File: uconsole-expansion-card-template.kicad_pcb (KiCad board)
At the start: 2 copper layers, 35.8 x 77 mm, 21 parts, among them U1 UC EXPANSION, U2 Speaker, U3 Speaker

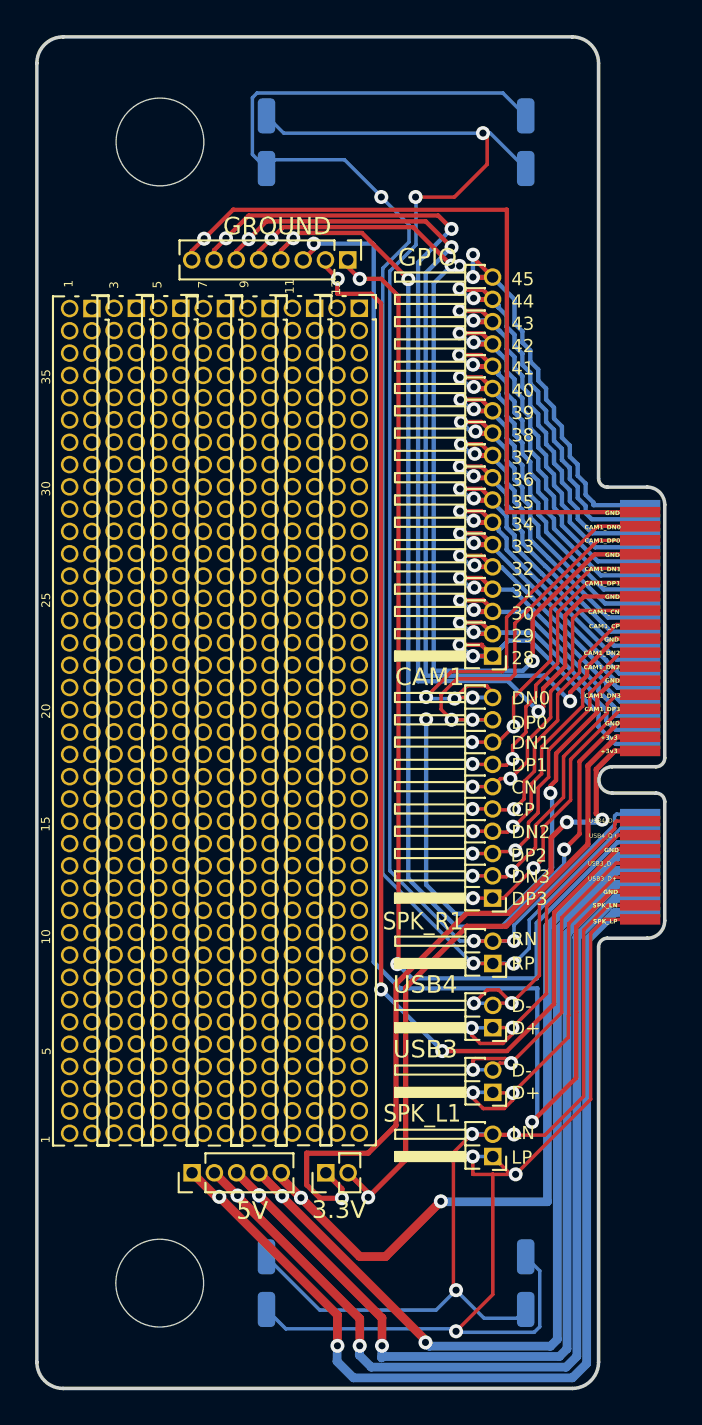
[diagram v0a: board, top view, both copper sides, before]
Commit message: Board 1.27mm passes to production!
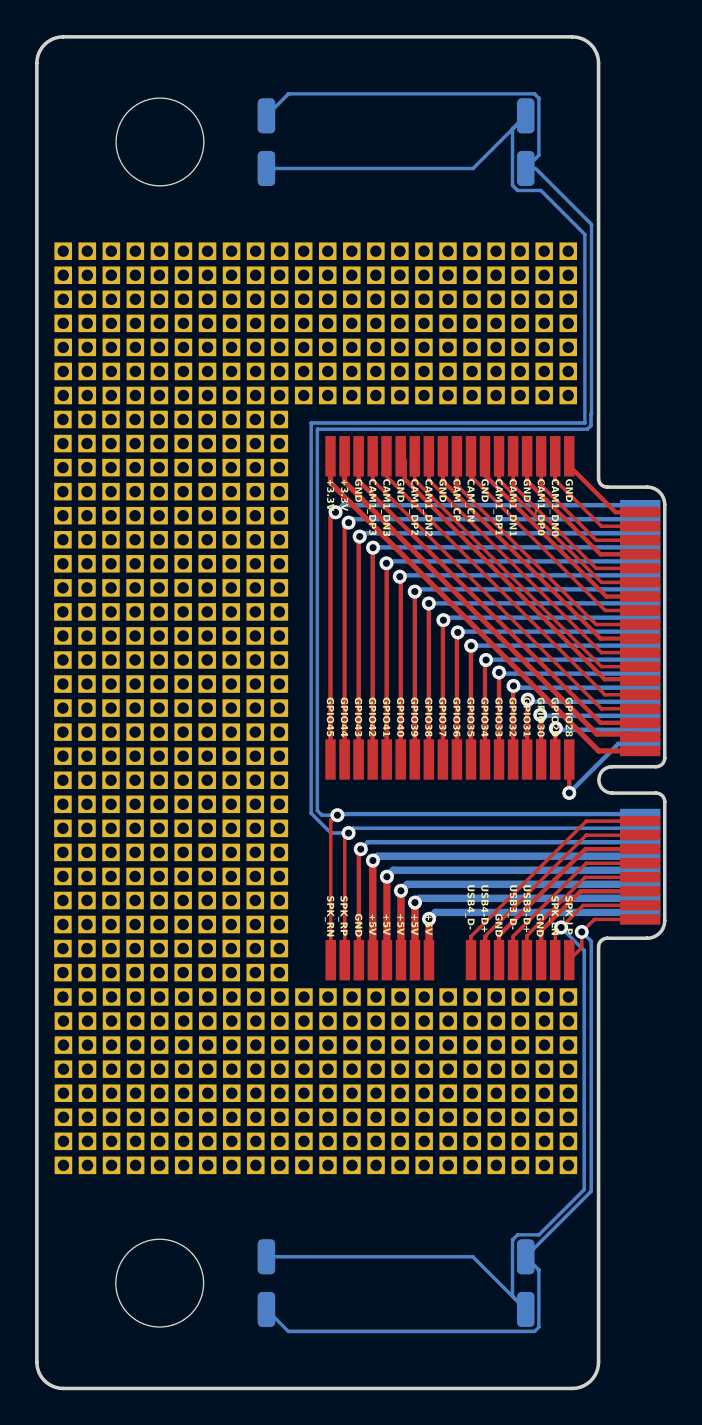
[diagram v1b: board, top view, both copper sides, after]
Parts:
- removed 1, 11, 13, 3, 5, 7, 9: PinSocket_2x38_P1.27mm_Vertical, Connector_PinSocket_1.27mm:PinSocket_2x38_P1.27mm_Vertical
- removed 3V1: Conn_01x02, Connector_PinHeader_1.27mm:PinHeader_1x02_P1.27mm_Vertical
- removed 5V1: Conn_01x05, Connector_PinHeader_1.27mm:PinHeader_1x05_P1.27mm_Vertical
- removed CAM1: Conn_01x10, Connector_PinHeader_1.27mm:PinHeader_1x10_P1.27mm_Horizontal
- removed GPIO1: Conn_01x18, Connector_PinHeader_1.27mm:PinHeader_1x18_P1.27mm_Horizontal
- removed GROUND1: Conn_01x08, Connector_PinHeader_1.27mm:PinHeader_1x08_P1.27mm_Vertical
- removed SPK_L1, SPK_R1, USB3, USB4: Conn_01x02, Connector_PinHeader_1.27mm:PinHeader_1x02_P1.27mm_Horizontal
- added ?: , , F.Cu at (111.0, 73.7)
- added ?: , , F.Cu at (90.5, 114.8)
- added ?: , , F.Cu at (87.7, 87.4)
- added ?: , , F.Cu at (89.1, 77.8)
- added ?: , , F.Cu at (102.0, 85.4)
- added ?: , , F.Cu at (94.6, 80.6)
- added ?: , , F.Cu at (87.7, 108.0)
- added ?: , , F.Cu at (83.6, 108.0)
- added ?: , , F.Cu at (89.1, 123.0)
- added ?: , , F.Cu at (95.9, 109.3)
- added ?: , , F.Cu at (93.2, 102.5)
- added ?: , , F.Cu at (94.6, 113.4)
- added ?: , , F.Cu at (83.6, 117.6)
- added ?: , , F.Cu at (90.5, 106.6)
- added ?: , , F.Cu at (98.7, 117.6)
- added ?: , , F.Cu at (108.4, 114.1)
- added ?: , , F.Cu at (95.9, 95.6)
- added ?: , , F.Cu at (90.5, 83.3)
- added ?: , , F.Cu at (112.4, 124.4)
- added ?: , , F.Cu at (83.6, 121.7)
- added ?: , , F.Cu at (87.7, 99.7)
- added ?: , , F.Cu at (85.0, 92.9)
- added ?: , , F.Cu at (86.3, 87.4)
- added ?: , , F.Cu at (85.0, 97.0)
- added ?: , , F.Cu at (101.4, 79.2)
- added ?: , , F.Cu at (94.6, 87.4)
- added ?: , , F.Cu at (93.2, 97.0)
- added ?: , , F.Cu at (93.2, 116.2)
- added ?: , , F.Cu at (95.9, 84.7)
- added ?: , , F.Cu at (83.6, 83.3)
- added ?: , , F.Cu at (111.0, 79.2)
- added ?: , , F.Cu at (98.7, 75.1)
- added ?: , , F.Cu at (86.3, 97.0)
- added ?: , , F.Cu at (86.3, 92.9)
- added ?: , , F.Cu at (94.6, 117.6)
- added ?: , , F.Cu at (91.8, 98.4)
- added ?: , , F.Cu at (93.2, 113.4)
- added ?: , , F.Cu at (91.8, 88.8)
- added ?: , , F.Cu at (94.6, 108.0)
- added ?: , , F.Cu at (100.1, 125.8)
- added ?: , , F.Cu at (90.5, 103.8)
- added ?: , , F.Cu at (87.7, 76.5)
- added ?: , , F.Cu at (91.8, 87.4)
- added ?: , , F.Cu at (83.6, 118.9)
- added ?: , , F.Cu at (94.6, 91.5)
- added ?: , , F.Cu at (98.7, 125.8)
- added ?: , , F.Cu at (109.7, 125.8)
- added ?: , , F.Cu at (87.7, 102.5)
- added ?: , , F.Cu at (100.1, 80.6)
- added ?: , , F.Cu at (87.7, 80.6)
- added ?: , , F.Cu at (105.2, 85.4)
- added ?: , , F.Cu at (111.0, 120.3)
- added ?: , , F.Cu at (85.0, 106.6)
- added ?: , , F.Cu at (87.7, 83.3)
- added ?: , , F.Cu at (85.0, 79.2)
- added ?: , , F.Cu at (95.9, 110.7)
- added ?: , , F.Cu at (94.6, 99.7)
- added ?: , , F.Cu at (112.4, 79.2)
- added ?: , , F.Cu at (89.1, 92.9)
- added ?: , , F.Cu at (106.9, 120.3)
- added ?: , , F.Cu at (94.6, 81.9)
- added ?: , , F.Cu at (93.2, 105.2)
- added ?: , , F.Cu at (86.4, 116.2)
- added ?: , , F.Cu at (83.6, 99.7)
- added ?: , , F.Cu at (87.7, 92.9)
- added ?: , , F.Cu at (90.5, 77.8)
- added ?: , , F.Cu at (85.0, 83.3)
- added ?: , , F.Cu at (109.6, 73.7)
- added ?: , , F.Cu at (108.3, 123.0)
- added ?: , , F.Cu at (93.2, 91.5)
- added ?: , , F.Cu at (102.8, 76.5)
- added ?: , , F.Cu at (104.2, 120.3)
- added ?: , , F.Cu at (86.3, 109.3)
- added ?: , , F.Cu at (83.6, 84.7)
- added ?: , , F.Cu at (112.4, 76.5)
- added ?: , , F.Cu at (83.6, 87.4)
- added ?: , , F.Cu at (109.6, 79.2)
- added ?: , , F.Cu at (94.6, 124.4)
- added ?: , , F.Cu at (91.8, 120.3)
- added ?: , , F.Cu at (101.4, 116.2)
- added ?: , , F.Cu at (86.3, 101.1)
- added ?: , , F.Cu at (104.2, 76.5)
- added ?: , , F.Cu at (90.5, 99.7)
- added ?: , , F.Cu at (106.9, 123.0)
- added ?: , , F.Cu at (105.5, 117.6)
- added ?: , , F.Cu at (95.9, 76.5)
- added ?: , , F.Cu at (85.0, 103.8)
- added ?: , , F.Cu at (90.5, 112.1)
- added ?: , , F.Cu at (97.3, 80.6)
- added ?: , , F.Cu at (85.0, 75.1)
- added ?: , , F.Cu at (91.8, 118.9)
- added ?: , , F.Cu at (112.4, 114.1)
- added ?: , , F.Cu at (91.8, 73.7)
- added ?: , , F.Cu at (85.0, 81.9)
- added ?: , , F.Cu at (102.8, 125.8)
- added ?: , , F.Cu at (104.2, 118.9)
- added ?: , , F.Cu at (93.2, 80.6)
- added ?: , , F.Cu at (101.4, 80.6)
- added ?: , , F.Cu at (101.4, 77.8)
- added ?: , , F.Cu at (104.2, 123.0)
- added ?: , , F.Cu at (85.0, 113.4)
- added ?: , , F.Cu at (86.3, 94.3)
- added ?: , , F.Cu at (112.4, 118.9)
- added ?: , , F.Cu at (94.6, 106.6)
- added ?: , , F.Cu at (85.0, 80.6)
- added ?: , , F.Cu at (111.0, 80.6)
- added ?: , , F.Cu at (90.5, 117.6)
- added ?: , , F.Cu at (87.7, 117.6)
- added ?: , , F.Cu at (94.6, 94.3)
- added ?: , , F.Cu at (106.9, 75.1)
- added ?: , , F.Cu at (100.1, 79.2)
- added ?: , , F.Cu at (86.4, 81.9)
- added ?: , , F.Cu at (101.4, 117.6)
- added ?: , , F.Cu at (94.6, 75.1)
- added ?: , , F.Cu at (90.5, 94.3)
- added ?: , , F.Cu at (105.5, 75.1)
- added ?: , , F.Cu at (93.2, 123.0)
- added ?: , , F.Cu at (94.6, 79.2)
- added ?: , , F.Cu at (87.7, 124.4)
- added ?: , , F.Cu at (89.1, 105.2)
- added ?: , , F.Cu at (94.6, 125.8)
- added ?: , , F.Cu at (105.5, 125.8)
- added ?: , , F.Cu at (93.2, 121.7)
- added ?: , , F.Cu at (105.5, 73.7)
- added ?: , , F.Cu at (95.9, 113.4)
- added ?: , , F.Cu at (97.3, 77.8)
- added ?: , , F.Cu at (83.6, 103.8)
- added ?: , , F.Cu at (95.9, 98.4)
- added ?: , , F.Cu at (87.7, 91.5)
- added ?: , , F.Cu at (90.5, 91.5)
- added ?: , , F.Cu at (91.8, 101.1)
- added ?: , , F.Cu at (103.6, 85.4)
- added ?: , , F.Cu at (100.1, 123.0)
- added ?: , , F.Cu at (101.4, 121.7)
- added ?: , , F.Cu at (83.6, 97.0)
- added ?: , , F.Cu at (85.0, 123.0)
- added ?: , , F.Cu at (95.9, 114.8)
- added ?: , , F.Cu at (98.7, 80.6)
- added ?: , , F.Cu at (90.5, 97.0)
- added ?: , , F.Cu at (95.9, 102.5)
- added ?: , , F.Cu at (85.0, 86.0)
- added ?: , , F.Cu at (106.9, 121.7)
- added ?: , , F.Cu at (108.3, 125.8)
- added ?: , , F.Cu at (89.1, 87.4)
- added ?: , , F.Cu at (106.0, 85.4)
- added ?: , , F.Cu at (100.4, 85.4)
- added ?: , , F.Cu at (93.2, 98.4)
- added ?: , , F.Cu at (89.1, 125.8)
- added ?: , , F.Cu at (89.1, 103.8)
- added ?: , , F.Cu at (91.8, 84.7)
- added ?: , , F.Cu at (91.8, 105.2)
- added ?: , , F.Cu at (94.6, 120.3)
- added ?: , , F.Cu at (83.6, 123.0)
- added ?: , , F.Cu at (112.4, 123.0)
- added ?: , , F.Cu at (106.9, 117.6)
- added ?: , , F.Cu at (89.1, 79.2)
- added ?: , , F.Cu at (108.4, 85.4)
- added ?: , , F.Cu at (105.5, 76.5)
- added ?: , , F.Cu at (86.3, 99.7)
- added ?: , , F.Cu at (97.3, 120.3)
- added ?: , , F.Cu at (91.8, 92.9)
- added ?: , , F.Cu at (106.9, 81.9)
- added ?: , , F.Cu at (95.9, 94.3)
- added ?: , , F.Cu at (108.3, 79.2)
- added ?: , , F.Cu at (90.5, 76.5)
- added ?: , , F.Cu at (86.3, 105.2)
- added ?: , , F.Cu at (90.5, 101.1)
- added ?: , , F.Cu at (87.7, 73.7)
- added ?: , , F.Cu at (109.2, 114.1)
- added ?: , , F.Cu at (102.8, 124.4)
- added ?: , , F.Cu at (91.8, 91.5)
- added ?: , , F.Cu at (91.8, 79.2)
- added ?: , , F.Cu at (93.2, 95.6)
- added ?: , , F.Cu at (97.3, 117.6)
- added ?: , , F.Cu at (90.5, 110.7)
- added ?: , , F.Cu at (85.0, 110.7)
- added ?: , , F.Cu at (89.1, 116.2)
- added ?: , , F.Cu at (91.8, 77.8)
- added ?: , , F.Cu at (85.0, 114.8)
- added ?: , , F.Cu at (86.3, 88.8)
- added ?: , , F.Cu at (97.3, 124.4)
- added ?: , , F.Cu at (89.1, 83.3)
- added ?: , , F.Cu at (94.6, 109.3)
- added ?: , , F.Cu at (91.8, 117.6)
- added ?: , , F.Cu at (108.3, 116.2)
- added ?: , , F.Cu at (108.3, 77.8)
- added ?: , , F.Cu at (97.3, 125.8)
- added ?: , , F.Cu at (96.0, 123.0)
- added ?: , , F.Cu at (109.6, 80.6)
- added ?: , , F.Cu at (89.1, 99.7)
- added ?: , , F.Cu at (87.7, 81.9)
- added ?: , , F.Cu at (90.5, 73.7)
- added ?: , , F.Cu at (96.0, 118.9)
- added ?: , , F.Cu at (94.6, 98.4)
- added ?: , , F.Cu at (93.2, 77.8)
- added ?: , , F.Cu at (100.1, 76.5)
- added ?: , , F.Cu at (90.5, 124.4)
- added ?: , , F.Cu at (111.0, 81.9)
- added ?: , , F.Cu at (112.4, 121.7)
- added ?: , , F.Cu at (97.3, 73.7)
- added ?: , , F.Cu at (93.2, 88.8)
- added ?: , , F.Cu at (83.6, 113.4)
- added ?: , , F.Cu at (109.6, 77.8)
- added ?: , , F.Cu at (87.7, 120.3)
- added ?: , , F.Cu at (89.1, 94.3)
- added ?: , , F.Cu at (87.7, 116.2)
- added ?: , , F.Cu at (97.3, 123.0)
- added ?: , , F.Cu at (104.2, 73.7)
- added ?: , , F.Cu at (112.4, 116.2)
- added ?: , , F.Cu at (112.4, 117.6)
- added ?: , , F.Cu at (91.8, 109.3)
- added ?: , , F.Cu at (100.1, 118.9)
- added ?: , , F.Cu at (111.6, 85.4)
- added ?: , , F.Cu at (107.6, 114.1)
- added ?: , , F.Cu at (111.0, 76.5)
- added ?: , , F.Cu at (106.9, 73.7)
- added ?: , , F.Cu at (93.2, 109.3)
- added ?: , , F.Cu at (86.3, 98.4)
- added ?: , , F.Cu at (94.6, 83.3)
- added ?: , , F.Cu at (109.7, 124.4)
- added ?: , , F.Cu at (90.5, 86.0)
- added ?: , , F.Cu at (91.8, 86.0)
- added ?: , , F.Cu at (93.2, 90.2)
- added ?: , , F.Cu at (90.5, 75.1)
- added ?: , , F.Cu at (109.7, 117.6)
- added ?: , , F.Cu at (87.7, 84.7)
- added ?: , , F.Cu at (95.9, 101.1)
- added ?: , , F.Cu at (89.1, 91.5)
- added ?: , , F.Cu at (94.6, 95.6)
- added ?: , , F.Cu at (111.0, 77.8)
- added ?: , , F.Cu at (91.8, 81.9)
- added ?: , , F.Cu at (95.9, 112.1)
- added ?: , , F.Cu at (86.4, 79.2)
- added ?: , , F.Cu at (83.6, 73.7)
- added ?: , , F.Cu at (104.2, 124.4)
- added ?: , , F.Cu at (102.8, 81.9)
- added ?: , , F.Cu at (95.9, 91.5)
- added ?: , , F.Cu at (93.2, 120.3)
- added ?: , , F.Cu at (87.7, 112.1)
- added ?: , , F.Cu at (87.7, 77.8)
- added ?: , , F.Cu at (95.9, 105.2)
- added ?: , , F.Cu at (102.8, 117.6)
- added ?: , , F.Cu at (105.5, 121.7)
- added ?: , , F.Cu at (98.8, 85.4)
- added ?: , , F.Cu at (102.8, 80.6)
- added ?: , , F.Cu at (108.3, 76.5)
- added ?: , , F.Cu at (86.3, 84.7)
- added ?: , , F.Cu at (83.6, 79.2)
- added ?: , , F.Cu at (89.1, 81.9)
- added ?: , , F.Cu at (94.6, 114.8)
- added ?: , , F.Cu at (111.0, 75.1)
- added ?: , , F.Cu at (96.0, 120.3)
- added ?: , , F.Cu at (83.6, 88.8)
- added ?: , , F.Cu at (83.6, 90.2)
- added ?: , , F.Cu at (90.5, 125.8)
- added ?: , , F.Cu at (93.2, 76.5)
- added ?: , , F.Cu at (100.1, 73.7)
- added ?: , , F.Cu at (98.7, 118.9)
- added ?: , , F.Cu at (94.6, 123.0)
- added ?: , , F.Cu at (86.3, 112.1)
- added ?: , , F.Cu at (83.6, 81.9)
- added ?: , , F.Cu at (85.0, 117.6)
- added ?: , , F.Cu at (85.0, 124.4)
- added ?: , , F.Cu at (83.6, 102.5)
- added ?: , , F.Cu at (89.1, 108.0)
- added ?: , , F.Cu at (83.6, 86.0)
- added ?: , , F.Cu at (95.9, 73.7)
- added ?: , , F.Cu at (94.6, 101.1)
- added ?: , , F.Cu at (89.1, 109.3)
- added ?: , , F.Cu at (110.8, 114.1)
- added ?: , , F.Cu at (98.7, 116.2)
- added ?: , , F.Cu at (94.6, 77.8)
- added ?: , , F.Cu at (89.1, 112.1)
- added ?: , , F.Cu at (89.1, 120.3)
- added ?: , , F.Cu at (112.4, 85.4)
- added ?: , , F.Cu at (85.0, 76.5)
- added ?: , , F.Cu at (95.9, 106.6)
- added ?: , , F.Cu at (85.0, 116.2)
- added ?: , , F.Cu at (83.6, 75.1)
- added ?: , , F.Cu at (86.3, 106.6)
- added ?: , , F.Cu at (100.1, 117.6)
- added ?: , , F.Cu at (109.2, 85.4)
- added ?: , , F.Cu at (85.0, 87.4)
- added ?: , , F.Cu at (91.8, 97.0)
- added ?: , , F.Cu at (93.2, 73.7)
- added ?: , , F.Cu at (86.3, 86.0)
- added ?: , , F.Cu at (107.6, 85.4)
- added ?: , , F.Cu at (97.3, 75.1)
- added ?: , , F.Cu at (87.7, 86.0)
- added ?: , , F.Cu at (94.6, 90.2)
- added ?: , , F.Cu at (86.3, 91.5)
- added ?: , , F.Cu at (96.0, 121.7)
- added ?: , , F.Cu at (108.3, 73.7)
- added ?: , , F.Cu at (106.9, 118.9)
- added ?: , , F.Cu at (90.5, 113.4)
- added ?: , , F.Cu at (93.2, 103.8)
- added ?: , , F.Cu at (90.5, 105.2)
- added ?: , , F.Cu at (89.1, 95.6)
- added ?: , , F.Cu at (90.5, 116.2)
- added ?: , , F.Cu at (85.0, 88.8)
- added ?: , , F.Cu at (89.1, 121.7)
- added ?: , , F.Cu at (108.3, 75.1)
- added ?: , , F.Cu at (85.0, 98.4)
- added ?: , , F.Cu at (100.1, 124.4)
- added ?: , , F.Cu at (109.7, 121.7)
- added ?: , , F.Cu at (93.2, 101.1)
- added ?: , , F.Cu at (95.9, 80.6)
- added ?: , , F.Cu at (93.2, 86.0)
- added ?: , , F.Cu at (83.6, 76.5)
- added ?: , , F.Cu at (105.5, 124.4)
- added ?: , , F.Cu at (89.1, 98.4)
- added ?: , , F.Cu at (102.8, 85.4)
- added ?: , , F.Cu at (93.2, 124.4)
- added ?: , , F.Cu at (94.6, 103.8)
- added ?: , , F.Cu at (85.0, 99.7)
- added ?: , , F.Cu at (96.0, 125.8)
- added ?: , , F.Cu at (95.9, 87.4)
- added ?: , , F.Cu at (111.0, 125.8)
- added ?: , , F.Cu at (100.1, 121.7)
- added ?: , , F.Cu at (109.6, 76.5)
- added ?: , , F.Cu at (86.3, 108.0)
- added ?: , , F.Cu at (100.1, 75.1)
- added ?: , , F.Cu at (91.8, 95.6)
- added ?: , , F.Cu at (89.1, 80.6)
- added ?: , , F.Cu at (104.2, 116.2)
- added ?: , , F.Cu at (91.8, 94.3)
- added ?: , , F.Cu at (100.1, 120.3)
- added ?: , , F.Cu at (90.5, 88.8)
- added ?: , , F.Cu at (86.3, 113.4)
- added ?: , , F.Cu at (87.7, 110.7)
- added ?: , , F.Cu at (83.6, 91.5)
- added ?: , , F.Cu at (101.4, 81.9)
- added ?: , , F.Cu at (106.9, 76.5)
- added ?: , , F.Cu at (94.6, 118.9)
- added ?: , , F.Cu at (105.5, 79.2)
- added ?: , , F.Cu at (98.7, 123.0)
- added ?: , , F.Cu at (85.0, 84.7)
- added ?: , , F.Cu at (86.3, 114.8)
- added ?: , , F.Cu at (89.1, 110.7)
- added ?: , , F.Cu at (104.4, 85.4)
- added ?: , , F.Cu at (83.6, 124.4)
- added ?: , , F.Cu at (94.6, 88.8)
- added ?: , , F.Cu at (89.1, 106.6)
- added ?: , , F.Cu at (85.0, 120.3)
- added ?: , , F.Cu at (101.4, 118.9)
- added ?: , , F.Cu at (91.8, 102.5)
- added ?: , , F.Cu at (97.3, 79.2)
- added ?: , , F.Cu at (85.0, 105.2)
- added ?: , , F.Cu at (95.9, 108.0)
- added ?: , , F.Cu at (94.6, 84.7)
- added ?: , , F.Cu at (105.5, 80.6)
- added ?: , , F.Cu at (91.8, 83.3)
- added ?: , , F.Cu at (91.8, 112.1)
- added ?: , , F.Cu at (102.8, 75.1)
- added ?: , , F.Cu at (89.1, 97.0)
- added ?: , , F.Cu at (87.7, 114.8)
- added ?: , , F.Cu at (87.7, 97.0)
- added ?: , , F.Cu at (102.8, 123.0)
- added ?: , , F.Cu at (98.7, 77.8)
- added ?: , , F.Cu at (94.6, 86.0)
- added ?: , , F.Cu at (108.3, 124.4)
- added ?: , , F.Cu at (109.7, 116.2)
- added ?: , , F.Cu at (89.1, 124.4)
- added ?: , , F.Cu at (83.6, 105.2)
- added ?: , , F.Cu at (90.5, 98.4)
- added ?: , , F.Cu at (96.0, 116.2)
- added ?: , , F.Cu at (102.8, 73.7)
- added ?: , , F.Cu at (105.5, 118.9)
- added ?: , , F.Cu at (94.6, 97.0)
- added ?: , , F.Cu at (108.3, 81.9)
- added ?: , , F.Cu at (101.4, 73.7)
- added ?: , , F.Cu at (83.6, 116.2)
- added ?: , , F.Cu at (90.5, 79.2)
- added ?: , , F.Cu at (111.0, 123.0)
- added ?: , , F.Cu at (94.6, 110.7)
- added ?: , , F.Cu at (85.0, 121.7)
- added ?: , , F.Cu at (111.0, 117.6)
- added ?: , , F.Cu at (93.2, 92.9)
- added ?: , , F.Cu at (90.5, 84.7)
- added ?: , , F.Cu at (85.0, 91.5)
- added ?: , , F.Cu at (95.9, 77.8)
- added ?: , , F.Cu at (86.4, 125.8)
- added ?: , , F.Cu at (83.6, 92.9)
- added ?: , , F.Cu at (85.0, 101.1)
- added ?: , , F.Cu at (106.9, 80.6)
- added ?: , , F.Cu at (94.6, 121.7)
- added ?: , , F.Cu at (93.2, 99.7)
- added ?: , , F.Cu at (87.7, 118.9)
- added ?: , , F.Cu at (104.2, 75.1)
- added ?: , , F.Cu at (102.8, 120.3)
- added ?: , , F.Cu at (86.3, 90.2)
- added ?: , , F.Cu at (101.4, 123.0)
- added ?: , , F.Cu at (98.7, 79.2)
- added ?: , , F.Cu at (105.5, 120.3)
- added ?: , , F.Cu at (91.8, 121.7)
- added ?: , , F.Cu at (95.9, 81.9)
- added ?: , , F.Cu at (95.9, 79.2)
- added ?: , , F.Cu at (87.7, 94.3)
- added ?: , , F.Cu at (98.7, 120.3)
- added ?: , , F.Cu at (98.7, 81.9)
- added ?: , , F.Cu at (86.4, 120.3)
- added ?: , , F.Cu at (86.4, 77.8)
- added ?: , , F.Cu at (89.1, 113.4)
- added ?: , , F.Cu at (93.2, 125.8)
- added ?: , , F.Cu at (86.4, 75.1)
- added ?: , , F.Cu at (90.5, 90.2)
- added ?: , , F.Cu at (93.2, 84.7)
- added ?: , , F.Cu at (87.7, 113.4)
- added ?: , , F.Cu at (105.5, 123.0)
- added ?: , , F.Cu at (104.2, 117.6)
- added ?: , , F.Cu at (91.8, 106.6)
- added ?: , , F.Cu at (104.2, 81.9)
- added ?: , , F.Cu at (96.0, 117.6)
- added ?: , , F.Cu at (87.7, 123.0)
- added ?: , , F.Cu at (83.6, 112.1)
- added ?: , , F.Cu at (93.2, 81.9)
- added ?: , , F.Cu at (83.6, 77.8)
- added ?: , , F.Cu at (87.7, 106.6)
- added ?: , , F.Cu at (111.6, 114.1)
- added ?: , , F.Cu at (109.7, 120.3)
- added ?: , , F.Cu at (102.8, 118.9)
- added ?: , , F.Cu at (91.8, 99.7)
- added ?: , , F.Cu at (110.8, 85.4)
- added ?: , , F.Cu at (93.2, 117.6)
- added ?: , , F.Cu at (101.4, 124.4)
- added ?: , , F.Cu at (86.3, 103.8)
- added ?: , , F.Cu at (98.7, 73.7)
- added ?: , , F.Cu at (101.4, 125.8)
- added ?: , , F.Cu at (108.3, 121.7)
- added ?: , , F.Cu at (101.4, 75.1)
- added ?: , , F.Cu at (104.2, 77.8)
- added ?: , , F.Cu at (95.9, 86.0)
- added ?: , , F.Cu at (89.1, 101.1)
- added ?: , , F.Cu at (83.6, 98.4)
- added ?: , , F.Cu at (86.4, 80.6)
- added ?: , , F.Cu at (108.3, 120.3)
- added ?: , , F.Cu at (95.9, 83.3)
- added ?: , , F.Cu at (85.0, 125.8)
- added ?: , , F.Cu at (87.7, 101.1)
- added ?: , , F.Cu at (90.5, 80.6)
- added ?: , , F.Cu at (102.8, 77.8)
- added ?: , , F.Cu at (90.5, 87.4)
- added ?: , , F.Cu at (85.0, 112.1)
- added ?: , , F.Cu at (85.0, 118.9)
- added ?: , , F.Cu at (93.2, 114.8)
- added ?: , , F.Cu at (112.4, 80.6)
- added ?: , , F.Cu at (100.1, 81.9)
- added ?: , , F.Cu at (91.8, 110.7)
- added ?: , , F.Cu at (85.0, 90.2)
- added ?: , , F.Cu at (95.9, 88.8)
- added ?: , , F.Cu at (106.9, 125.8)
- added ?: , , F.Cu at (105.5, 116.2)
- added ?: , , F.Cu at (86.4, 76.5)
- added ?: , , F.Cu at (89.1, 88.8)
- added ?: , , F.Cu at (102.8, 79.2)
- added ?: , , F.Cu at (98.7, 121.7)
- added ?: , , F.Cu at (91.8, 76.5)
- added ?: , , F.Cu at (112.4, 120.3)
- added ?: , , F.Cu at (111.0, 118.9)
- added ?: , , F.Cu at (106.9, 116.2)
- added ?: , , F.Cu at (111.0, 121.7)
- added ?: , , F.Cu at (106.9, 77.8)
- added ?: , , F.Cu at (90.5, 123.0)
- added ?: , , F.Cu at (104.2, 125.8)
- added ?: , , F.Cu at (101.4, 76.5)
- added ?: , , F.Cu at (87.7, 88.8)
- added ?: , , F.Cu at (93.2, 87.4)
- added ?: , , F.Cu at (85.0, 102.5)
- added ?: , , F.Cu at (112.4, 77.8)
- added ?: , , F.Cu at (90.5, 102.5)
- added ?: , , F.Cu at (101.2, 85.4)
- added ?: , , F.Cu at (91.8, 90.2)
- added ?: , , F.Cu at (90.5, 108.0)
- added ?: , , F.Cu at (97.3, 118.9)
- added ?: , , F.Cu at (93.2, 112.1)
- added ?: , , F.Cu at (91.8, 116.2)
- added ?: , , F.Cu at (87.7, 95.6)
- added ?: , , F.Cu at (85.0, 77.8)
- added ?: , , F.Cu at (87.7, 125.8)
- added ?: , , F.Cu at (97.3, 76.5)
- added ?: , , F.Cu at (99.6, 85.4)
- added ?: , , F.Cu at (95.9, 75.1)
- added ?: , , F.Cu at (89.1, 118.9)
- added ?: , , F.Cu at (89.1, 90.2)
- added ?: , , F.Cu at (87.7, 79.2)
- added ?: , , F.Cu at (106.8, 85.4)
- added ?: , , F.Cu at (91.8, 125.8)
- added ?: , , F.Cu at (89.1, 102.5)
- added ?: , , F.Cu at (112.4, 75.1)
- added ?: , , F.Cu at (94.6, 105.2)
- added ?: , , F.Cu at (93.2, 94.3)
- added ?: , , F.Cu at (111.0, 124.4)
- added ?: , , F.Cu at (83.6, 114.8)
- added ?: , , F.Cu at (106.9, 124.4)
- added ?: , , F.Cu at (85.0, 109.3)
- added ?: , , F.Cu at (90.5, 118.9)
- added ?: , , F.Cu at (108.3, 80.6)
- added ?: , , F.Cu at (91.8, 123.0)
- added ?: , , F.Cu at (97.3, 81.9)
- added ?: , , F.Cu at (100.1, 77.8)
- added ?: , , F.Cu at (86.3, 95.6)
- added ?: , , F.Cu at (86.4, 123.0)
- added ?: , , F.Cu at (90.5, 92.9)
- added ?: , , F.Cu at (87.7, 98.4)
- added ?: , , F.Cu at (89.1, 114.8)
- added ?: , , F.Cu at (112.4, 81.9)
- added ?: , , F.Cu at (108.3, 118.9)
- added ?: , , F.Cu at (94.6, 73.7)
- added ?: , , F.Cu at (86.4, 118.9)
- added ?: , , F.Cu at (95.9, 92.9)
- added ?: , , F.Cu at (85.0, 95.6)
- added ?: , , F.Cu at (93.2, 79.2)
- added ?: , , F.Cu at (93.2, 118.9)
- added ?: , , F.Cu at (86.3, 102.5)
- added ?: , , F.Cu at (91.8, 80.6)
- added ?: , , F.Cu at (83.6, 110.7)
- added ?: , , F.Cu at (90.5, 109.3)
- added ?: , , F.Cu at (98.7, 76.5)
- added ?: , , F.Cu at (95.9, 90.2)
- added ?: , , F.Cu at (83.6, 125.8)
- added ?: , , F.Cu at (87.7, 109.3)
- added ?: , , F.Cu at (105.5, 81.9)
- added ?: , , F.Cu at (91.8, 75.1)
- added ?: , , F.Cu at (83.6, 80.6)
- added ?: , , F.Cu at (93.2, 75.1)
- added ?: , , F.Cu at (100.1, 116.2)
- added ?: , , F.Cu at (91.8, 124.4)
- added ?: , , F.Cu at (109.7, 123.0)
- added ?: , , F.Cu at (90.5, 95.6)
- added ?: , , F.Cu at (97.3, 121.7)
- added ?: , , F.Cu at (94.6, 102.5)
- added ?: , , F.Cu at (86.4, 124.4)
- added ?: , , F.Cu at (94.6, 92.9)
- added ?: , , F.Cu at (105.5, 77.8)
- added ?: , , F.Cu at (85.0, 108.0)
- added ?: , , F.Cu at (86.4, 121.7)
- added ?: , , F.Cu at (83.6, 94.3)
- added ?: , , F.Cu at (97.3, 116.2)
- added ?: , , F.Cu at (98.7, 124.4)
- added ?: , , F.Cu at (93.2, 83.3)
- added ?: , , F.Cu at (87.7, 121.7)
- added ?: , , F.Cu at (109.6, 75.1)
- added ?: , , F.Cu at (94.6, 76.5)
- added ?: , , F.Cu at (102.8, 121.7)
- added ?: , , F.Cu at (112.4, 73.7)
- added ?: , , F.Cu at (89.1, 76.5)
- added ?: , , F.Cu at (86.4, 73.7)
- added ?: , , F.Cu at (87.7, 105.2)
- added ?: , , F.Cu at (102.8, 116.2)
- added ?: , , F.Cu at (83.6, 101.1)
- added ?: , , F.Cu at (89.1, 86.0)
- added ?: , , F.Cu at (87.7, 90.2)
- added ?: , , B.Cu at (99.6, 102.7)
- added ?: , , B.Cu at (100.4, 102.7)
- added ?: , , B.Cu at (108.4, 102.7)
- added ?: , , F.Cu at (95.9, 97.0)
- added ?: , , F.Cu at (83.6, 109.3)
- added ?: , , B.Cu at (110.0, 102.7)
- added ?: , , B.Cu at (104.4, 102.7)
- added ?: , , B.Cu at (104.5, 114.1)
- added ?: , , B.Cu at (106.0, 102.7)
- added ?: , , B.Cu at (112.4, 102.7)
- added ?: , , B.Cu at (102.9, 114.1)
- added ?: , , B.Cu at (107.6, 102.7)
- added ?: , , B.Cu at (102.1, 114.1)
- added ?: , , B.Cu at (99.7, 114.1)
- added ?: , , B.Cu at (105.2, 102.7)
- added ?: , , F.Cu at (86.3, 83.3)
- added ?: , , B.Cu at (106.8, 102.7)
- added ?: , , B.Cu at (110.8, 102.7)
- added ?: , , B.Cu at (103.6, 102.7)
- added ?: , , B.Cu at (100.5, 114.1)
- added ?: , , B.Cu at (101.2, 102.7)
- added ?: , , B.Cu at (102.8, 102.7)
- added ?: , , B.Cu at (102.0, 102.7)
- added ?: , , B.Cu at (98.9, 114.1)
- added ?: , , B.Cu at (111.6, 102.7)
- added ?: , , B.Cu at (103.7, 114.1)
- added ?: , , F.Cu at (86.4, 117.6)
- added ?: , , B.Cu at (109.2, 102.7)
- added ?: , , B.Cu at (101.3, 114.1)
- added ?: , , F.Cu at (90.5, 81.9)
- added ?: , , F.Cu at (83.6, 106.6)
- added ?: , , F.Cu at (91.8, 108.0)
- added ?: , , F.Cu at (91.8, 114.8)
- added ?: , , F.Cu at (93.2, 110.7)
- added ?: , , F.Cu at (89.1, 73.7)
- added ?: , , F.Cu at (93.2, 108.0)
- added ?: , , F.Cu at (94.6, 116.2)
- added ?: , , F.Cu at (91.8, 113.4)
- added ?: , , F.Cu at (104.2, 121.7)
- added ?: , , F.Cu at (101.4, 120.3)
- added ?: , , F.Cu at (112.4, 125.8)
- added ?: , , F.Cu at (89.1, 84.7)
- added ?: , , F.Cu at (86.3, 110.7)
- added ?: , , F.Cu at (83.6, 95.6)
- added ?: , , F.Cu at (89.1, 75.1)
- added ?: , , F.Cu at (87.7, 103.8)
- added ?: , , F.Cu at (108.3, 117.6)
- added ?: , , F.Cu at (104.2, 80.6)
- added ?: , , F.Cu at (104.2, 79.2)
- added ?: , , F.Cu at (95.9, 103.8)
- added ?: , , F.Cu at (109.7, 118.9)
- added ?: , , F.Cu at (94.6, 112.1)
- added ?: , , F.Cu at (83.6, 120.3)
- added ?: , , F.Cu at (96.0, 124.4)
- added ?: , , F.Cu at (109.6, 81.9)
- added ?: , , F.Cu at (111.0, 116.2)
- added ?: , , F.Cu at (85.0, 73.7)
- added ?: , , F.Cu at (90.5, 120.3)
- added ?: , , F.Cu at (90.5, 121.7)
- added ?: , , F.Cu at (91.8, 103.8)
- added ?: , , F.Cu at (110.0, 114.1)
- added ?: , , F.Cu at (106.8, 114.1)
- added ?: , , F.Cu at (106.9, 79.2)
- added ?: , , F.Cu at (87.7, 75.1)
- added ?: , , F.Cu at (95.9, 99.7)
- added ?: , , F.Cu at (93.2, 106.6)
- added ?: , , F.Cu at (89.1, 117.6)
- added ?: , , F.Cu at (85.0, 94.3)
- added ?: , , F.Cu at (110.0, 85.4)
- added GPIO45: , , B.Cu at (98.8, 102.7)
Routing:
- net GND: track 518.5 -> 129.4 mm, vias 23 -> 1
- net +5V: track 259.1 -> 89.4 mm, vias 10 -> 5
- net +3V3: track 79.2 -> 49.8 mm, vias 4 -> 0
- net /CAM1_DN0: track 27.1 -> 8.64 mm, vias 3 -> 0
- net /SPEAKER_RN: track 83.8 -> 101.5 mm, vias 4 -> 1
- net /CAM1_DP0: track 23.0 -> 8.59 mm, vias 2 -> 0
- net /GPIO29: track 19.9 -> 6.63 mm, vias 2 -> 1
- net /USB3_D+: track 22.2 -> 9.22 mm, vias 2 -> 0
- net /GPIO28: track 19.5 -> 7.10 mm, vias 2 -> 1
- net /GPIO30: track 19.0 -> 8.27 mm, vias 2 -> 1
- net /USB3_D-: track 20.7 -> 10.3 mm, vias 2 -> 0
- net /SPEAKER_RP: track 91.1 -> 100.9 mm, vias 3 -> 1
- net /GPIO31: track 17.7 -> 9.87 mm, vias 2 -> 1
- net /SPEAKER_LP: track 55.5 -> 47.9 mm, vias 3 -> 1
- net /GPIO45: track 24.6 -> 31.7 mm, vias 2 -> 1
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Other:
- board text added: "+3.3V"
- board text added: "CAM1_DP2"
- board text added: "CAM_CN"
- board text added: "CAM_CP"
- board text added: "USB3-D+"
- board text added: "USB4-D+"
- board text added: "Yébedeh's uConsole Universal Expansion Board v0.3"
- board text removed: "+3v3"
- board text removed: "1"
- board text removed: "10"
- board text removed: "15"
- board text removed: "20"
- board text removed: "25"
- board text removed: "28"
- board text removed: "29"
- board text removed: "3.3V"
- board text removed: "30"
- board text removed: "31"
- board text removed: "32"
- board text removed: "33"
- board text removed: "34"
- board text removed: "35"
- board text removed: "36"
- board text removed: "37"
- board text removed: "38"
- board text removed: "39"
- board text removed: "40"
- board text removed: "41"
- board text removed: "42"
- board text removed: "43"
- board text removed: "44"
- board text removed: "45"
- board text removed: "5"
- board text removed: "5V"
- board text removed: "CAM1_CN"
- board text removed: "CAM1_CP"
- board text removed: "CN"
- board text removed: "CP"
- board text removed: "D+"
- board text removed: "D-"
- board text removed: "DN0"
- board text removed: "DN1"
- board text removed: "DN2"
- board text removed: "DN3"
- board text removed: "DP0"
- board text removed: "DP1"
- board text removed: "DP2"
- board text removed: "DP3"
- board text removed: "GPIO"
- board text removed: "GROUND"
- board text removed: "LN"
- board text removed: "LP"
- board text removed: "RN"
- board text removed: "RP"
- board text removed: "USB3_D+"
- board text removed: "USB4_D+"
- board text removed: "Yébedeh's uConsole Universal Expansion Board v0.2"
